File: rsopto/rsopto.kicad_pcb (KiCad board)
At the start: 2 copper layers, 4 parts, among them J1 DB9_Female, J2 HFBR-1515BZ

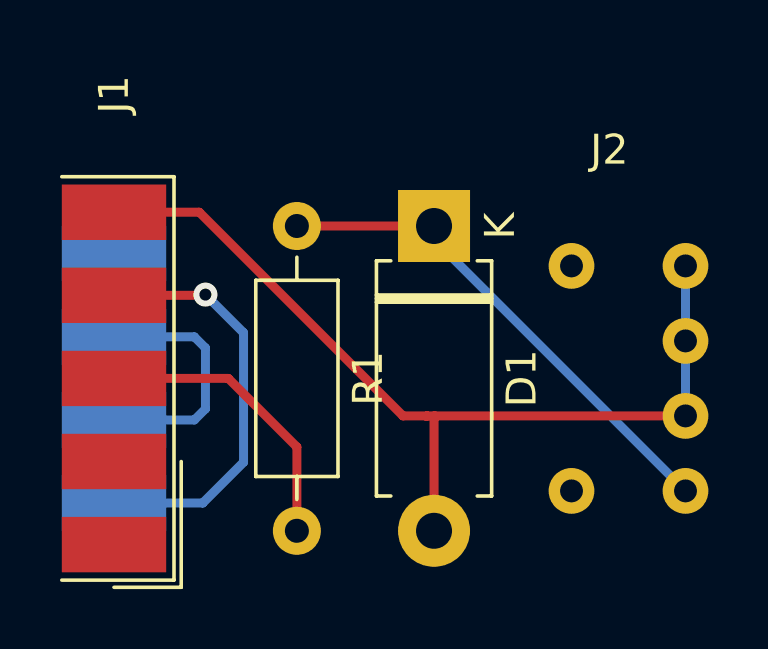
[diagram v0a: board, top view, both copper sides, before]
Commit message: Fix structure
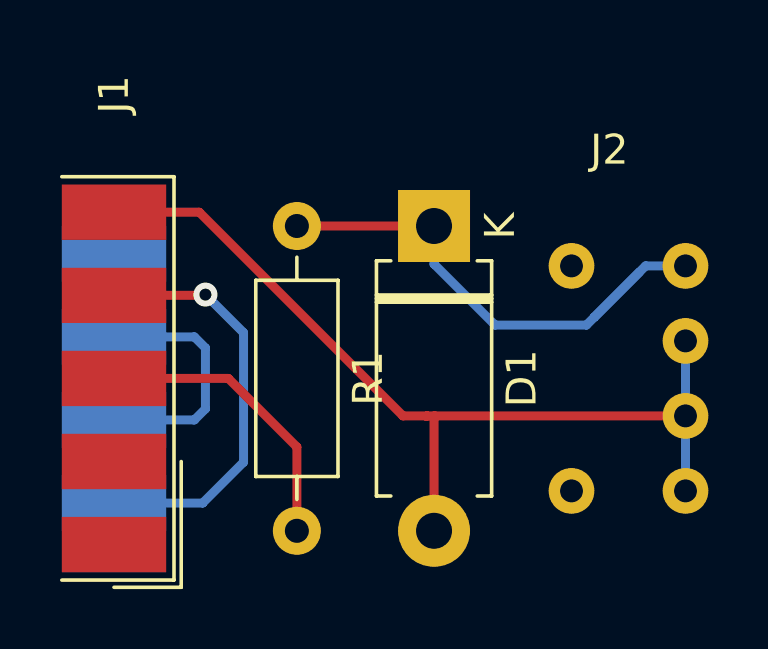
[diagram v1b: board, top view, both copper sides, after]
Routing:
- net Net-(D1-Pad1): track 18.0 -> 19.2 mm
